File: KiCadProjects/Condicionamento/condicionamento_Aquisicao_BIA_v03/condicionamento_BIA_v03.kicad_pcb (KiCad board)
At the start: 2 copper layers, 90 x 100 mm, 27 parts, among them J1 Vref, J2 tensoes, J3 sinais analogicos, J4 comunicacao / sinais digitais, J5 sinais_condicionados, J6 alimetacao_Master, J7 Eletrodos, U1 AD828AN, U2 BluePill_STM32F103C, U3 BluePill_STM32F103C

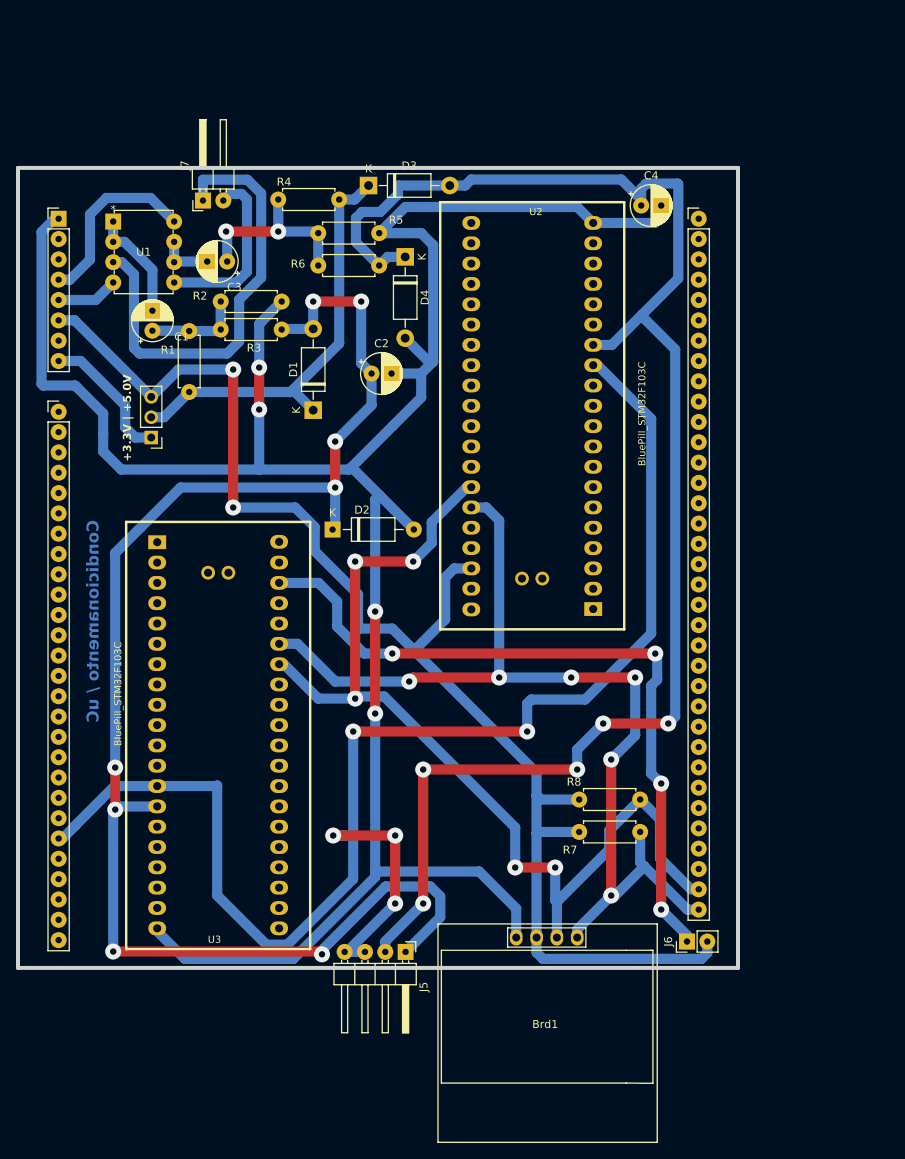
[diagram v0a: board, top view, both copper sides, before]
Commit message: baseado barramento v04
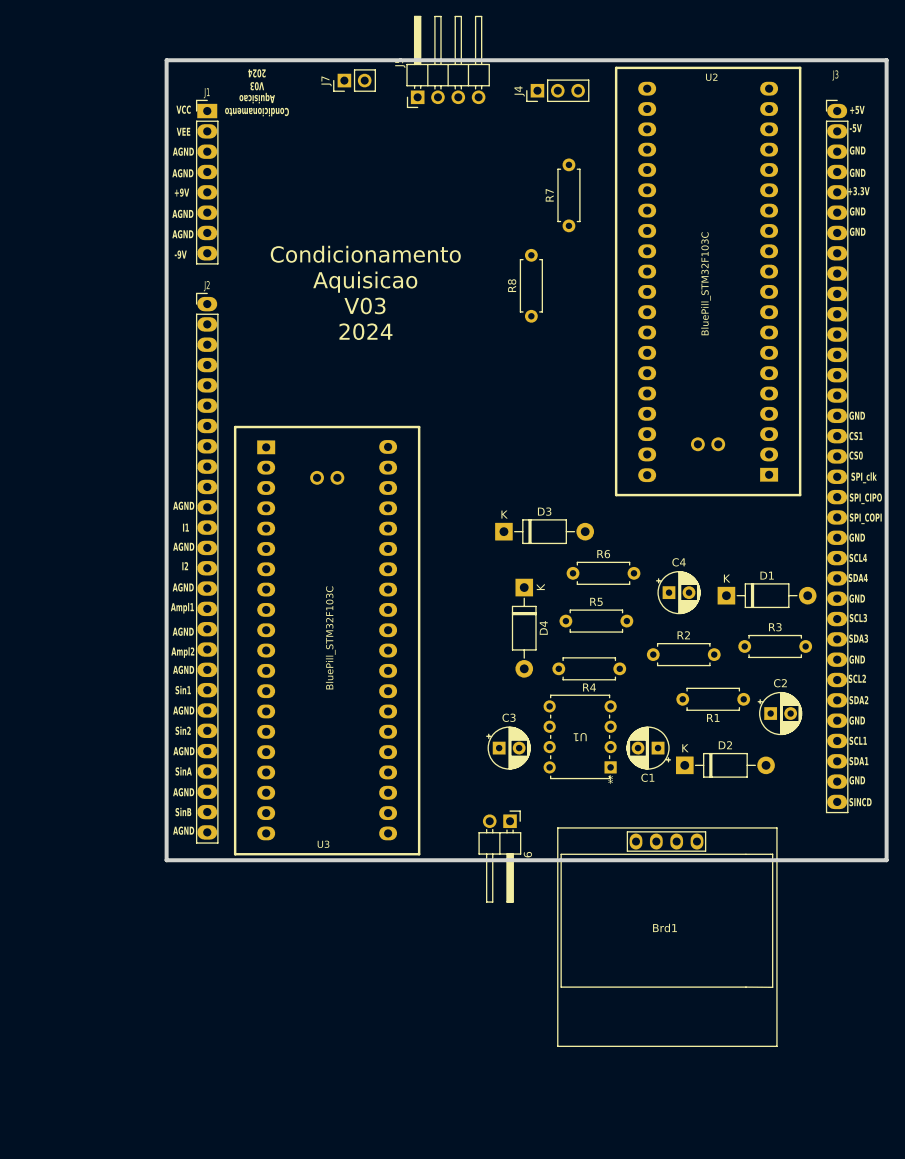
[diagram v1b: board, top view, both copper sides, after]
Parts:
- Brd1: footprint OLED_i2c:128x64OLED -> OLED:128x64OLED
- J1: value Vref -> alimentacao analogica; footprint Connector_PinHeader_2.54mm:PinHeader_1x03_P2.54mm_Vertical -> Connector_PinHeader_2.54mm:PinHeader_1x08_P2.54mm_Vertical
- J2: value tensoes -> sinais analogicos; footprint Connector_PinHeader_2.54mm:PinHeader_1x08_P2.54mm_Vertical -> Connector_PinHeader_2.54mm:PinHeader_1x27_P2.54mm_Vertical
- J3: value sinais analogicos -> comunicacao / sinais digitais; footprint Connector_PinHeader_2.54mm:PinHeader_1x27_P2.54mm_Vertical -> Connector_PinHeader_2.54mm:PinHeader_1x35_P2.54mm_Vertical
- J4: value comunicacao / sinais digitais -> Vref; footprint Connector_PinHeader_2.54mm:PinHeader_1x35_P2.54mm_Vertical -> Connector_PinHeader_2.54mm:PinHeader_1x03_P2.54mm_Vertical
- J6: value alimetacao_Master -> Eletrodos; footprint Connector_PinHeader_2.54mm:PinHeader_1x02_P2.54mm_Vertical -> Connector_PinHeader_2.54mm:PinHeader_1x02_P2.54mm_Horizontal
- J7: value Eletrodos -> alimetacao_Master; footprint Connector_PinHeader_2.54mm:PinHeader_1x02_P2.54mm_Horizontal -> Connector_PinHeader_2.54mm:PinHeader_1x02_P2.54mm_Vertical
- U1: footprint AD828:N_8_ADI -> AD828:AD828
- U2, U3: footprint STM32_Bluepill:BluePill_STM32F103C -> BluePill_STM32:BluePill_STM32F103C
- moved J5 106.8 mm to (138.5, 39.7), turned to 90 degrees
- moved J3 104.3 mm to (190.9, 41.4)
- moved U1 92.3 mm to (162.6, 123.4), turned to 180 degrees
- moved C1 82.0 mm to (168.5, 121.0), turned to 180 degrees
- moved R1 79.2 mm to (179.2, 114.9), turned to 180 degrees
- moved R3 76.6 mm to (179.3, 108.3)
- moved R7 76.3 mm to (157.4, 55.7), turned to 90 degrees
- moved R2 69.8 mm to (167.9, 109.3)
- moved C3 69.7 mm to (148.6, 121.0), turned to 0 degrees
- moved R4 68.3 mm to (163.7, 111.1)
- moved C2 65.5 mm to (182.6, 116.7)
- moved R8 61.9 mm to (152.7, 67.0), turned to 90 degrees
- moved R5 57.5 mm to (157.0, 105.1)
- moved D1 56.6 mm to (177.1, 102.0), turned to 0 degrees
- moved D2 53.0 mm to (171.8, 123.2)
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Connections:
- net AmpI2 renamed SCL4
- J1 pad 1: +3.3V -> VCC
- J1 pad 2: Vref -> VEE
- J1 pad 3: +5V -> Earth
- J2 pad 1: Earth -> unconnected-(J2-Pin_1-Pad1)
- J2 pad 2: VCC -> unconnected-(J2-Pin_2-Pad2)
- J2 pad 3: VEE -> unconnected-(J2-Pin_3-Pad3)
- J2 pad 4: +9V -> unconnected-(J2-Pin_4-Pad4)
- J2 pad 5: -9V -> unconnected-(J2-Pin_5-Pad5)
- J2 pad 6: +5V -> unconnected-(J2-Pin_6-Pad6)
- J2 pad 7: -5V -> unconnected-(J2-Pin_7-Pad7)
- J2 pad 8: +3.3V -> unconnected-(J2-Pin_8-Pad8)
- J3 pad 1: unconnected-(J3-Pin_1-Pad1) -> +5V
- J3 pad 16: unconnected-(J3-Pin_16-Pad16) -> Earth
- J3 pad 17: unconnected-(J3-Pin_17-Pad17) -> CS1
- J3 pad 18: unconnected-(J3-Pin_18-Pad18) -> CS0
- J3 pad 19: unconnected-(J3-Pin_19-Pad19) -> SPI_clk
- J3 pad 2: unconnected-(J3-Pin_2-Pad2) -> -5V
- J3 pad 20: I1 -> SPI_CIPO
- J3 pad 21: I2 -> SPI_COPI
- J3 pad 22: AmpI1 -> Earth
- J3 pad 24: Sin1 -> SDA4
- J3 pad 25: Sin2 -> Earth
- J3 pad 26: SinA -> SCL3
- J3 pad 27: SinB -> SDA3
- J3 pad 3: unconnected-(J3-Pin_3-Pad3) -> Earth
- J3 pad 4: unconnected-(J3-Pin_4-Pad4) -> Earth
- J3 pad 5: unconnected-(J3-Pin_5-Pad5) -> +3.3V
- J3 pad 6: unconnected-(J3-Pin_6-Pad6) -> Earth
- J3 pad 7: unconnected-(J3-Pin_7-Pad7) -> Earth
- J4 pad 1: SINC -> +3.3V
- J4 pad 2: SPI_COPI -> Vref
- J4 pad 3: SPI_CIPO -> +5V
- J6 pad 1: Net-(J6-Pin_1) -> E1
- J6 pad 2: +5V -> E2
- J7 pad 1: E1 -> Net-(J7-Pin_1)
- J7 pad 2: E2 -> +5V
- U3 pad 38: Net-(J6-Pin_1) -> Net-(J7-Pin_1)
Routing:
- net Earth: track 292.0 -> 0.00 mm, vias 4 -> 0
- net Amp_E2: track 196.1 -> 0.00 mm, vias 5 -> 0
- net AmpI1: track 189.1 -> 0.00 mm, vias 5 -> 0
- net Amp_E1: track 184.8 -> 0.00 mm, vias 8 -> 0
- net +5V: track 171.8 -> 0.00 mm, vias 2 -> 0
- net SCL1: track 126.0 -> 0.00 mm, vias 5 -> 0
- net SDA1: track 124.9 -> 0.00 mm, vias 6 -> 0
- net Net-(J6-Pin_1): track 90.8 -> 0.00 mm, vias 4 -> 0
- net E1: track 57.0 -> 0.00 mm
- net Vref: track 53.7 -> 0.00 mm
- net nó4: track 23.6 -> 0.00 mm, vias 2 -> 0
- net +9V: track 23.2 -> 0.00 mm
- net E2: track 22.3 -> 0.00 mm
- net +3.3V: track 17.1 -> 0.00 mm
- net nó1: track 14.0 -> 0.00 mm
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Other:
- board text added: "+3.3V"
- board text added: "+5V"
- board text added: "+9V"
- board text added: "-5V"
- board text added: "-9V"
- board text added: "AGND"
- board text added: "Ampl1"
- board text added: "Ampl2"
- board text added: "CS0"
- board text added: "CS1"
- board text added: "Condicionamento Aquisicao V03 2024"
- board text added: "GND"
- board text added: "I1"
- board text added: "I2"
- board text added: "SCL1"
- board text added: "SCL2"
- board text added: "SCL3"
- board text added: "SCL4"
- board text added: "SDA1"
- board text added: "SDA2"
- board text added: "SDA3"
- board text added: "SDA4"
- board text added: "SINCD"
- board text added: "SPI_CIPO"
- board text added: "SPI_COPI"
- board text added: "SPI_clk"
- board text added: "Sin1"
- board text added: "Sin2"
- board text added: "SinA"
- board text added: "SinB"
- board text added: "VCC"
- board text added: "VEE"
- board text removed: "+3.3V | +5.0V"
- board text removed: "Condicionamento / uC"
- board text removed: "Condicionamento / uC V01 - 2023"
